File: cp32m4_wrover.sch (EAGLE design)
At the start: 30 parts, among them Q3 DMG341, U2 AP2112-3.3, X2 32.768

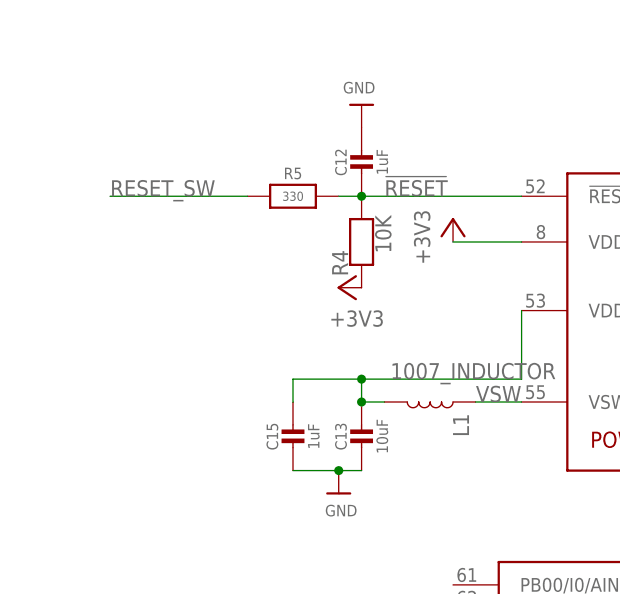
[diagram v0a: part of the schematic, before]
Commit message: routing done-ish, ground airwires
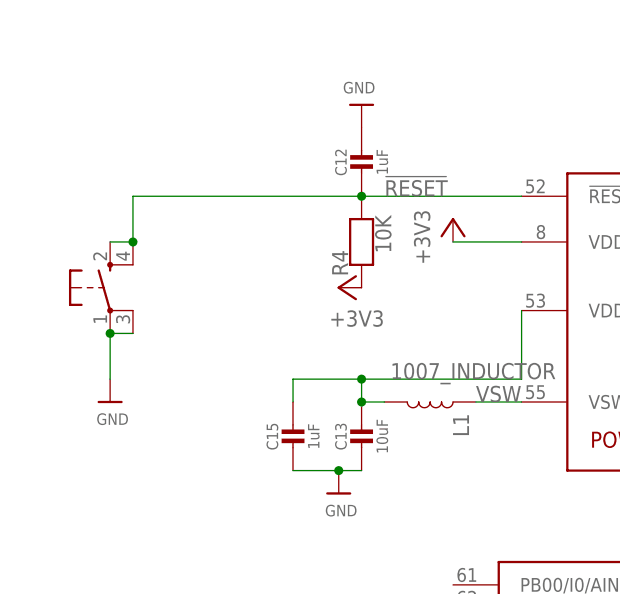
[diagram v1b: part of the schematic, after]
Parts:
- removed R5: 330, microbuilder:RESISTOR_0603_NOOUT
- added SW1: SPST_TACT-KMR2, adafruit:SPST_TACT-KMR2
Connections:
- net !RESET: now also SW1.S, SW1.S1; no longer R5.1
- net GND: now also SW1.P, SW1.P1
- net RESET_SW: no longer R5.2
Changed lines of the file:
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@@
 <part name="+3V1" library="supply1" library_urn="urn:adsk.eagle:library:371" deviceset="+3V3" device=""/>
 <part name="U$7" library="00_bsiepert" library_urn="urn:adsk.eagle:library:6622413" deviceset="ESP32_WROVER" device=""/>
-<part name="R5" library="microbuilder" deviceset="RESISTOR" device="_0603_NOOUT" value="330"/>
 <part name="U$50" library="00_bsiepert" deviceset="AMPHENOL_MICRO_USB" device="AMPHENOL_MICRO_USB_BETTER"/>
+<part name="SW1" library="adafruit" library_urn="urn:adsk.eagle:library:420" deviceset="SPST_TACT" device="-KMR2" package3d_urn="urn:adsk.eagle:package:6240885/1"/>
+<part name="U$1" library="microbuilder" deviceset="GND" device=""/>
 </parts>
 <sheets>
@@
 </instance>
 <instance part="U$7" gate="G$1" x="304.8" y="96.52" smashed="yes"/>
-<instance part="R5" gate="G$1" x="33.02" y="160.02" smashed="yes" rot="MR0">
-<attribute name="NAME" x="33.02" y="162.56" size="1.27" layer="95" font="vector" rot="MR0" align="center"/>
-<attribute name="VALUE" x="33.02" y="160.02" size="1.016" layer="96" font="vector" ratio="15" rot="MR0" align="center"/>
-</instance>
 <instance part="U$50" gate="G$1" x="297.18" y="226.06" smashed="yes" rot="R180"/>
+<instance part="SW1" gate="G$1" x="12.7" y="149.86" smashed="yes"/>
+<instance part="U$1" gate="G$1" x="12.7" y="137.16" smashed="yes">
+<attribute name="VALUE" x="11.176" y="134.62" size="1.27" layer="96"/>
+</instance>
 </instances>
 <busses>
@@
 <label x="373.38" y="157.48" size="1.778" layer="95" align="bottom-right"/>
 </segment>
+<segment>
+<pinref part="SW1" gate="G$1" pin="P1"/>
+<pinref part="SW1" gate="G$1" pin="P"/>
+<wire x1="15.24" y1="144.78" x2="12.7" y2="144.78" width="0.1524" layer="91"/>
+<pinref part="U$1" gate="G$1" pin="GND"/>
+<wire x1="12.7" y1="144.78" x2="12.7" y2="139.7" width="0.1524" layer="91"/>
+<junction x="12.7" y="144.78"/>
+</segment>
 </net>
 <net name="AREF" class="0">
@@
 <pinref part="U$14" gate="G$3" pin="!RESET"/>
 <wire x1="58.42" y1="160.02" x2="40.64" y2="160.02" width="0.1524" layer="91"/>
-<wire x1="38.1" y1="160.02" x2="40.64" y2="160.02" width="0.1524" layer="91"/>
-<pinref part="R5" gate="G$1" pin="1"/>
+<pinref part="SW1" gate="G$1" pin="S1"/>
+<wire x1="40.64" y1="160.02" x2="15.24" y2="160.02" width="0.1524" layer="91"/>
+<wire x1="15.24" y1="160.02" x2="15.24" y2="154.94" width="0.1524" layer="91"/>
+<pinref part="SW1" gate="G$1" pin="S"/>
+<wire x1="15.24" y1="154.94" x2="12.7" y2="154.94" width="0.1524" layer="91"/>
+<junction x="15.24" y="154.94"/>
 </segment>
 </net>
@@
 <pinref part="U$44" gate="G$1" pin="RESET"/>
 <wire x1="332.74" y1="233.68" x2="315.1124" y2="233.68" width="0.1524" layer="91"/>
-</segment>
-<segment>
-<pinref part="R5" gate="G$1" pin="2"/>
-<wire x1="12.7" y1="160.02" x2="27.94" y2="160.02" width="0.1524" layer="91"/>
-<label x="12.7" y="160.02" size="1.778" layer="95"/>
 </segment>
 </net>
@@
 will not be understood (or retained) with this version.
 </note>
+<note version="8.3" severity="warning">
+Since Version 8.3, EAGLE supports the association of 3D packages
+with devices in libraries, schematics, and board files. Those 3D
+packages will not be understood (or retained) with this version.
+</note>
 <note version="9.0" severity="warning">
